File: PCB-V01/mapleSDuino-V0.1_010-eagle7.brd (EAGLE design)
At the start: 82 x 27 mm, 11 parts, among them IC2 LAN-USR-ES1

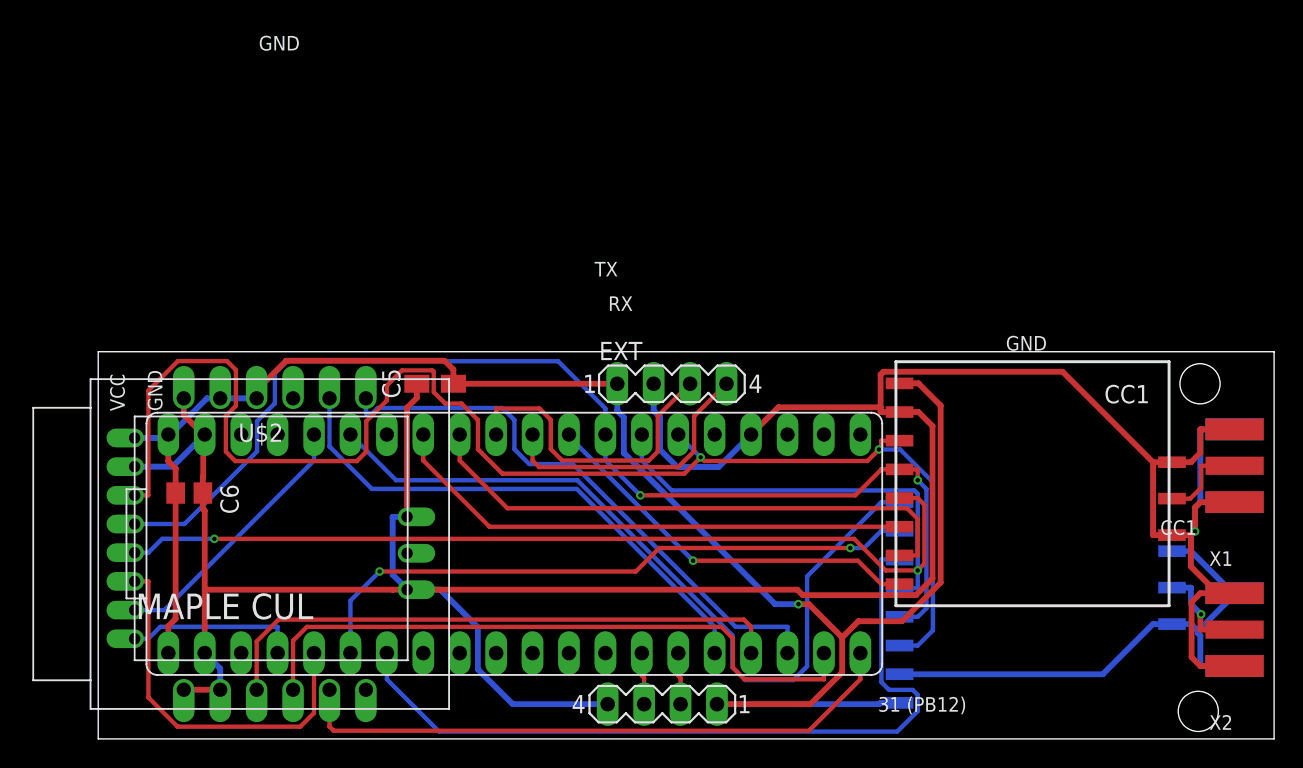
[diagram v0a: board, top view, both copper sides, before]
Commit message: V010
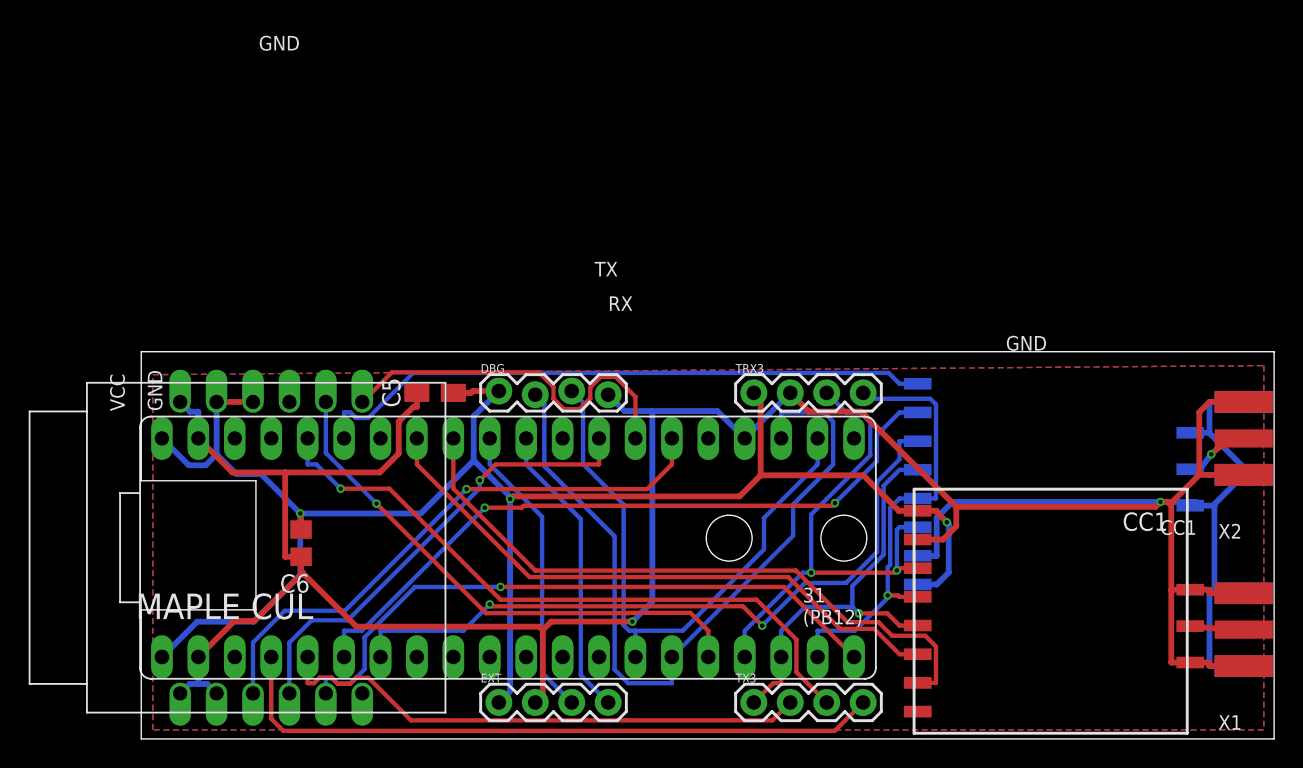
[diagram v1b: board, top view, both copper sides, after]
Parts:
- removed U$2: CC1101_MODULE1DIL_BIG, CC1101:CC1101_MODULE1_DIL-2
- added TRX3, TX3: (no value), SparkFun-Connectors:1X04
- DBG: device con-lstb:MA04-1 -> SparkFun-Connectors:1X04_LOCK
- EXT: device con-lstb:MA04-1 -> SparkFun-Connectors:1X04
- moved EXT 25.3 mm to (27.9, 2.54)
- moved DBG 24.5 mm to (27.9, 24.1), turned to 0 degrees
- moved X2 13.4 mm to (81.9, 21.0)
- moved X1 11.4 mm to (81.9, 7.62)
- moved CC1 8.98 mm to (57.1, 1.91)
- moved C6 8.54 mm to (14.1, 13.7), turned to 270 degrees
- moved CC2 8.35 mm to (57.1, 24.8)
- moved C5 0.64 mm to (23.5, 24.1)
- moved U$1 0.52 mm to (28.6, 13.3)
- moved IC2 0.36 mm to (11.4, 13.3)
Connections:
- net WIZ_CS renamed SS2
- removed net N$33: IC2.6
- removed net RST: IC2.3, U$1.17
- removed net RX_DBG: DBG.3, U$1.14
- removed net TX_DBG: DBG.2, U$1.15
- new net MOSI2: CC1.MOSI, CC2.MOSI, TRX3.3, U$1.17
- new net SS1: U$1.29
- net CC_CS0: no longer U$1.29
- net CC_CS2: now also TX3.4; no longer U$2.8
- net CC_IN_2: now also TX3.2; no longer U$2.6
- net CC_OUT_2: now also TX3.3; no longer U$2.7
- net GND: now also TRX3.2; no longer U$2.11, U$2.2, U$2.9
- net MISO1: now also IC2.7; no longer CC1.MISO, CC2.MISO, U$2.5
- net MISO2: now also CC1.MISO, CC2.MISO, TX3.1; no longer IC2.7
- net MOSI1: now also IC2.3; no longer CC1.MOSI, CC2.MOSI, U$2.3
- net RX1: now also DBG.3, U$1.14
- net SCK1: now also IC2.4; no longer CC1.SCLK, CC2.SCLK, U$2.4
- net SCK2: now also CC1.SCLK, CC2.SCLK, TRX3.4; no longer IC2.4
- net TX1: now also DBG.2, U$1.15
- net VCC: now also TRX3.1; no longer U$2.1
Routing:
- net MISO1: track 92.5 -> 26.3 mm, vias 2 -> 0
- net MOSI1: track 99.7 -> 39.7 mm, vias 2 -> 1
- net TX1: track 0.00 -> 54.4 mm
- net SCK1: track 80.6 -> 32.4 mm, vias 2 -> 1
- net RX1: track 0.00 -> 41.2 mm
- net RST: track 40.5 -> 0.00 mm
- net MOSI2: track 0.00 -> 36.2 mm, vias 0 -> 2
- net CC_CS2: track 12.1 -> 46.8 mm
- net GND: track 263.3 -> 230.5 mm, vias 1 -> 2
- net CC_OUT_2: track 18.6 -> 46.2 mm, vias 0 -> 1
- net CC_CS0: track 27.5 -> 0.00 mm, vias 1 -> 0
- net SCK2: track 45.4 -> 31.6 mm, vias 0 -> 1
- net CC_CS1: track 55.5 -> 43.6 mm
- net CC_IN_2: track 26.0 -> 37.7 mm
- net MISO2: track 40.0 -> 29.1 mm, vias 0 -> 1
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- added copper zone on layer 1, net GND
- added copper zone on layer 16, net GND
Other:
- board size 82 x 27 mm -> 79 x 27 mm
